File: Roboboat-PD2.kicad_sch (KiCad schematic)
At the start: 37 parts, among them J1 12V, J10 Motor, J11 Motor, J12 Motor, J13 Motor, J15 14.4V, J17 PGOOD TP, J18 GND TP, J19 PGOOD, J2 Bucky, J3 Jetson, J4 Motor, J5 Motor, J6 Motor, J7 Motor, J8 Motor, J9 Motor, SW1 Jumper, U1 AOZ2379QI

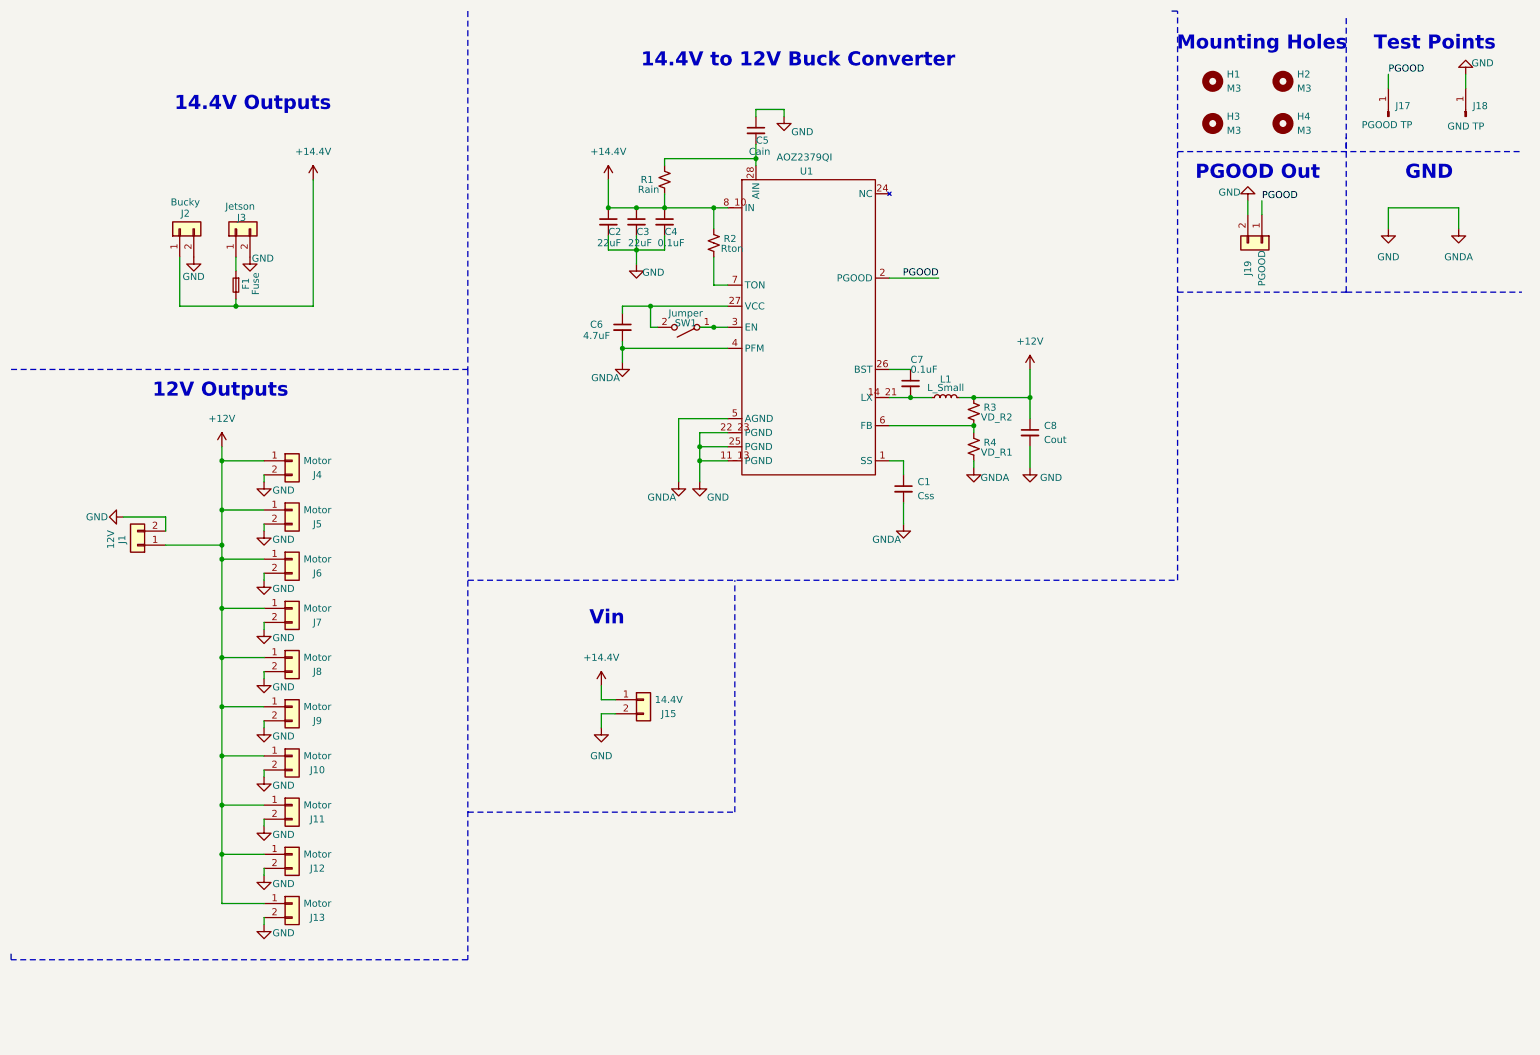
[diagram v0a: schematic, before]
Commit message: rearrange schematic
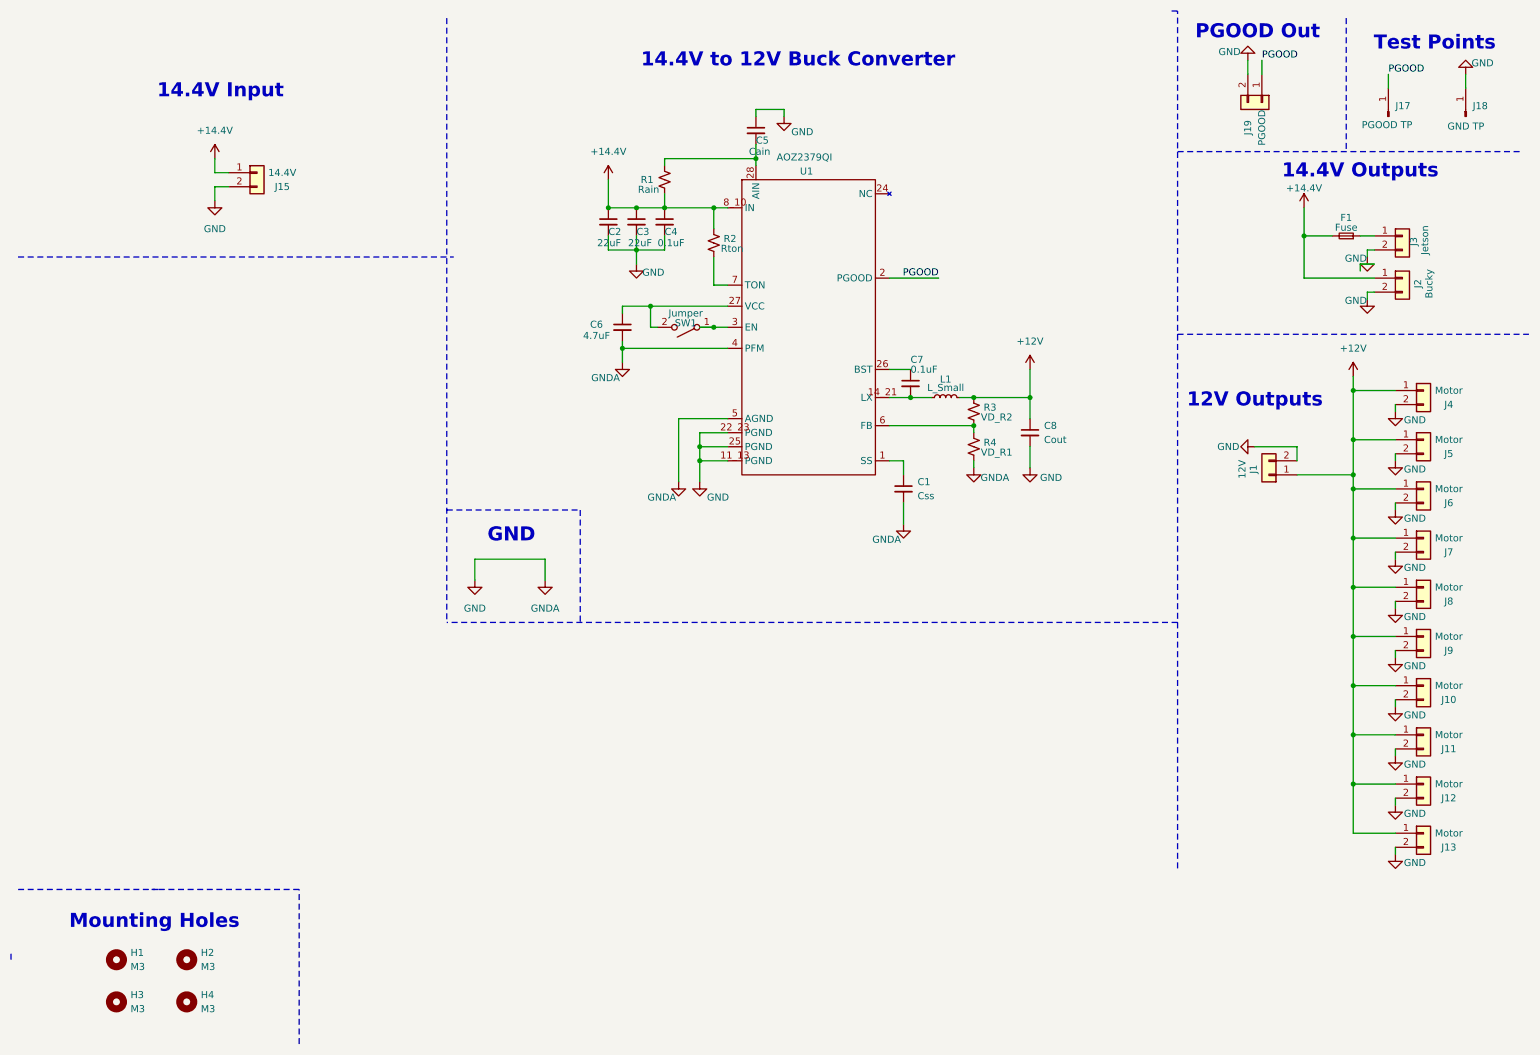
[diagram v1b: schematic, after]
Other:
- note added: "14.4V Input"
- note removed: "Vin"
- moved on the sheet: F1, H1, H2, H3, H4, J1, J10, J11, J12, J13, J15, J19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
